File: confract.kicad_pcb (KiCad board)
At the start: 2 copper layers, 117.1 x 81 mm, 44 parts, among them J1 Conn_01x05, J10 GS2, J11 Conn_01x04, J12 GS2, J13 GS2, J14 GS2, J15 GS2, J16 Conn_01x02, J2 GS3, J3 Conn_01x05, J4 GS3, J5 Audio-Jack-4, J6 GS2, J7 GS2, J8 GS2, J9 GS3, Q1 Q_NMOS_GSD, SW1 SW_Push, SW10 SW_Push, SW11 SW_Push, SW12 SW_Push, SW13 SW_Push, SW14 SW_Push, SW15 SW_Push, SW16 SW_Push, SW17 SW_Push, SW2 SW_Push, SW3 SW_Push, SW4 SW_Push, SW5 SW_Push, SW6 SW_Push, SW7 SW_Push, SW8 SW_Push, SW9 SW_Push, U1 MCP23017_QFN

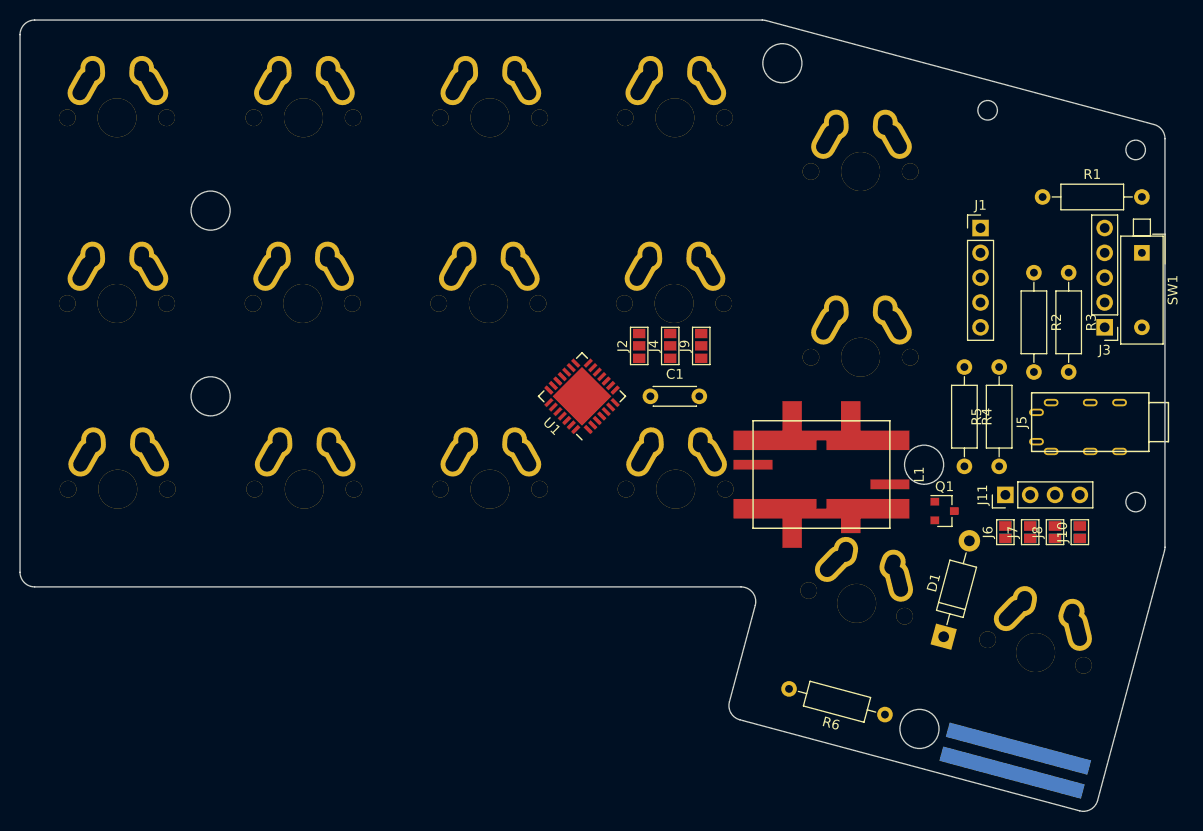
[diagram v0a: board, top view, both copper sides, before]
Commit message: update schematic and pcb
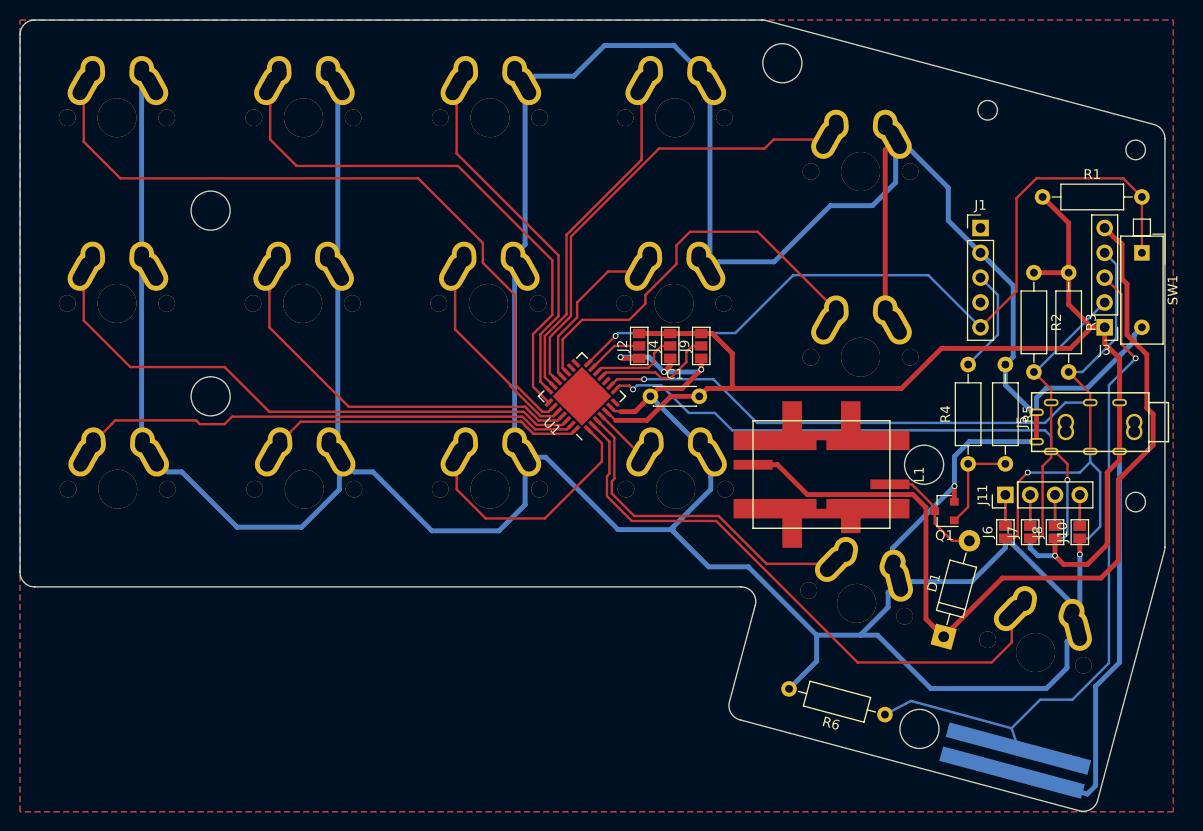
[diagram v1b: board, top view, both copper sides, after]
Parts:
- moved R5 10.4 mm to (170.8, 95.2), turned to 270 degrees
- moved R4 9.91 mm to (167.0, 105.4), turned to 90 degrees
- turned Q1 to 180 degrees
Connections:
- U1 pad 2: SW13 -> SW15
- U1 pad 4: SW15 -> SW13
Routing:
- net GND: track 0.00 -> 490.1 mm, vias 0 -> 5
- net VCC: track 0.00 -> 168.2 mm, vias 0 -> 1
- net SDA: track 0.00 -> 102.3 mm, vias 0 -> 2
- net VBUS: track 0.00 -> 92.2 mm
- net SCL: track 0.00 -> 89.0 mm, vias 0 -> 2
- net RESET: track 0.00 -> 81.0 mm, vias 0 -> 1
- net SW0: track 0.00 -> 72.0 mm
- net Press: track 0.00 -> 70.5 mm, vias 0 -> 1
- net SW15: track 0.00 -> 60.4 mm
- net SW5: track 0.00 -> 59.1 mm
- net SW1: track 0.00 -> 55.5 mm
- net SW10: track 0.00 -> 51.0 mm
- net SW4: track 0.00 -> 46.4 mm
- net SW9: track 0.00 -> 41.1 mm
- net SW6: track 0.00 -> 39.8 mm
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- added copper zone on B.Cu, net GND
- added copper zone on F.Cu, net GND
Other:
- net class Power added: clearance 0.2, trace_width 0.5, via_dia 0.6, via_drill 0.4
- rule trace_min: 0.2 -> 0.25
